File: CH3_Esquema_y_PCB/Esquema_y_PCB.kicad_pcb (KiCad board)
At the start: 2 copper layers, 143.4 x 83.7 mm, 45 parts, among them Q1 BC547, Q10 BC857, Q2 BC547, Q3 BC547, Q4 BC547, Q5 IRF9Z34N, Q7 BC547, Q9 BC857, U1 TL431LP, U2 LM358

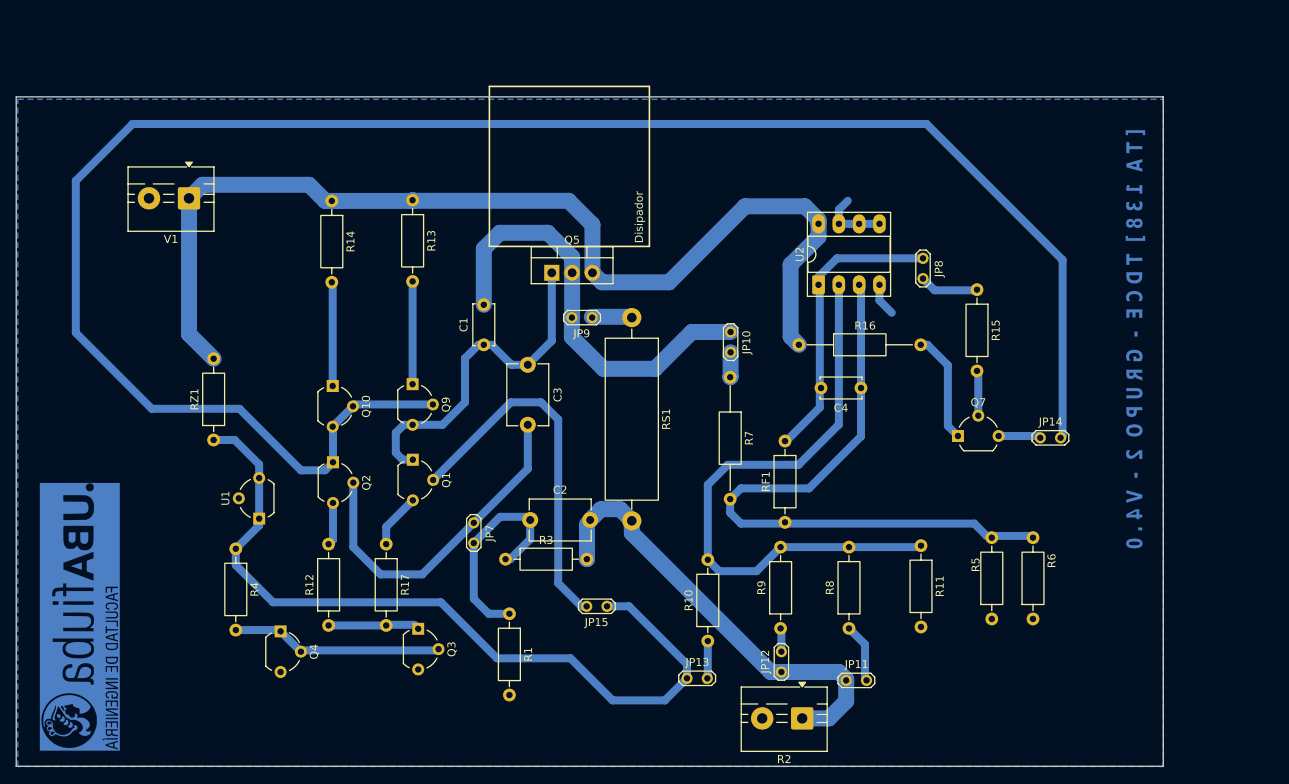
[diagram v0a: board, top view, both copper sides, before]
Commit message: Add files via upload
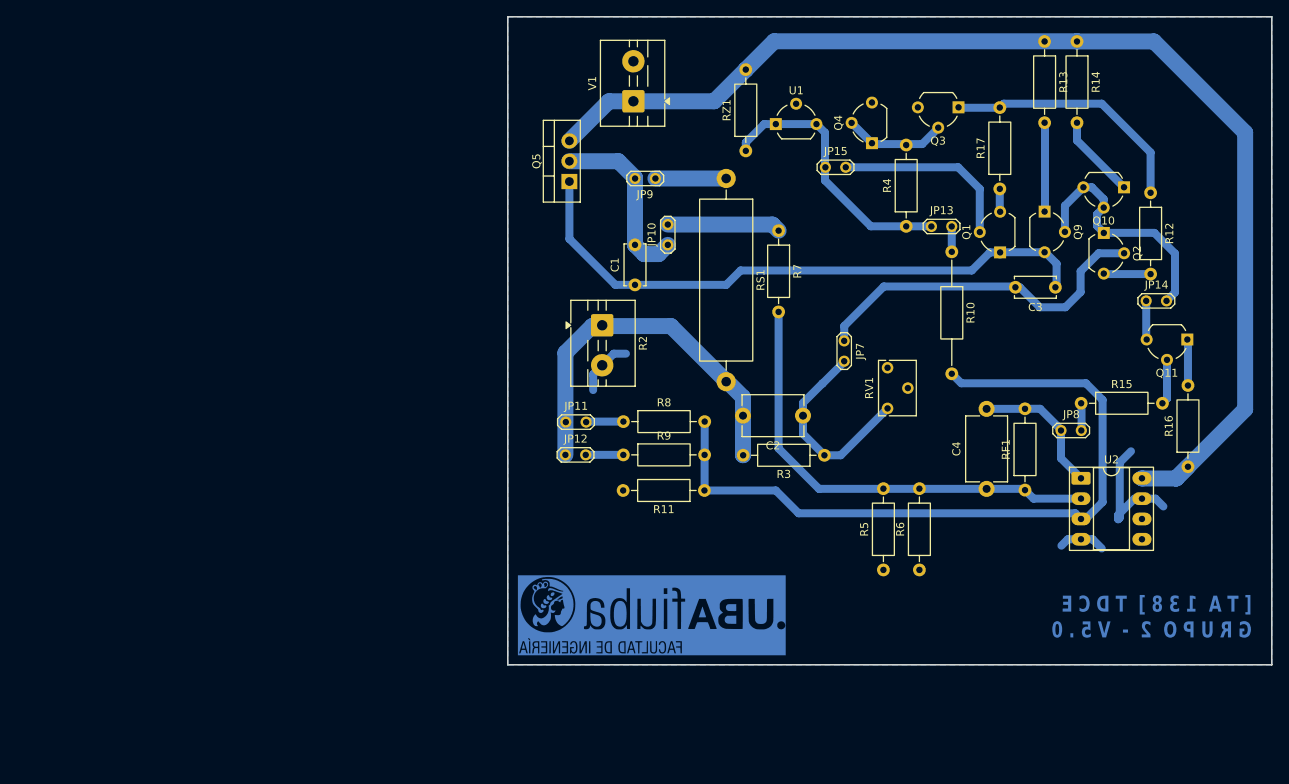
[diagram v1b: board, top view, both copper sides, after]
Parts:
- removed Q7: BC547, Package_TO_SOT_THT:TO-92_Wide
- removed R1: 10k, Resistor_THT:R_Axial_DIN0207_L6.3mm_D2.5mm_P10.16mm_Horizontal
- added Q11: BC557, Package_TO_SOT_THT:TO-92_Wide, F.Cu at (214.9, 90.3)
- added RV1: R_Potentiometer, Potentiometer_THT:Potentiometer_Bourns_3266W_Vertical, F.Cu at (177.5, 93.9)
- C3: footprint Capacitor_THT:C_Disc_D7.5mm_W5.0mm_P7.50mm -> Capacitor_THT:C_Disc_D5.0mm_W2.5mm_P5.00mm
- C4: footprint Capacitor_THT:C_Disc_D5.0mm_W2.5mm_P5.00mm -> Capacitor_THT:C_Disc_D8.0mm_W5.0mm_P10.00mm
- Q10, Q9: value BC857 -> BC557
- R10: footprint Resistor_THT:R_Axial_DIN0207_L6.3mm_D2.5mm_P10.16mm_Horizontal -> Resistor_THT:R_Axial_DIN0207_L6.3mm_D2.5mm_P15.24mm_Horizontal
- R16, R7: footprint Resistor_THT:R_Axial_DIN0207_L6.3mm_D2.5mm_P15.24mm_Horizontal -> Resistor_THT:R_Axial_DIN0207_L6.3mm_D2.5mm_P10.16mm_Horizontal
- moved R12 116.1 mm to (210.3, 72.0), turned to -90 degrees
- moved Q10 102.0 mm to (207.0, 71.3), turned to 180 degrees
- moved Q2 100.5 mm to (204.5, 77.0)
- moved Q4 95.9 mm to (175.5, 65.8), turned to 90 degrees
- moved R14 95.3 mm to (201.2, 53.1)
- moved Q3 93.9 mm to (186.3, 61.3), turned to 180 degrees
- moved R4 93.0 mm to (179.8, 76.2), turned to 90 degrees
- moved R17 88.6 mm to (191.5, 71.5), turned to 90 degrees
- moved Q9 81.9 mm to (197.1, 74.3)
- moved R13 81.5 mm to (197.1, 53.1)
- moved U1 81.3 mm to (163.5, 63.4), turned to 0 degrees
- moved Q1 77.8 mm to (191.5, 79.5), turned to 90 degrees
- moved RZ1 75.7 mm to (159.8, 66.8)
- moved G*** 71.5 mm to (148.0, 124.8), turned to 180 degrees
- moved C3 66.7 mm to (198.4, 83.8), turned to 180 degrees
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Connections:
- C4 pad 1: Net-(U2A-+) -> Net-(U2A--)
- R10 pad 2: Net-(U2A--) -> Net-(U2A-+)
- R11 pad 1: Net-(U2A--) -> Net-(U2A-+)
- R5 pad 2: Net-(U2A-+) -> Net-(U2A--)
- R6 pad 2: Net-(U2A-+) -> Net-(U2A--)
- R7 pad 2: Net-(U2A-+) -> Net-(U2A--)
- R8 pad 2: Net-(U2A--) -> Net-(U2A-+)
- R9 pad 2: Net-(U2A--) -> Net-(U2A-+)
- RF1 pad 1: Net-(U2A-+) -> Net-(U2A--)
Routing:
- net /VB: track 232.5 -> 30.9 mm
- net /in: track 100.0 -> 34.0 mm
- net Net-(Q1-C): track 43.1 -> 76.0 mm
- net /drain: track 53.6 -> 22.5 mm
- net Net-(JP15-B): track 45.8 -> 23.2 mm
- net Net-(Q3-C): track 11.4 -> 32.0 mm
- net Net-(JP8-A): track 36.5 -> 17.5 mm
- net Net-(U2A--): track 74.9 -> 57.5 mm
- net GND: track 12.6 -> 29.6 mm
- net VCC: track 131.5 -> 147.5 mm
- net Net-(U2A-+): track 79.5 -> 93.7 mm
- net Net-(Q3-B): track 26.5 -> 12.7 mm
- net Net-(JP10-B): track 3.13 -> 14.2 mm
- net /out: track 56.9 -> 47.3 mm
- net Net-(Q11-E): track 13.8 -> 5.77 mm
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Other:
- board size 143.4 x 83.7 mm -> 95.5 x 81 mm
- board text added: "[ T A 1 3 8 ] T D C E G R U P O 2 - V 5 . 0"
- board text removed: "[ T A 1 3 8 ] T D C E - G R U P O 2 - V 4 . 0"

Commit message: Add files via upload
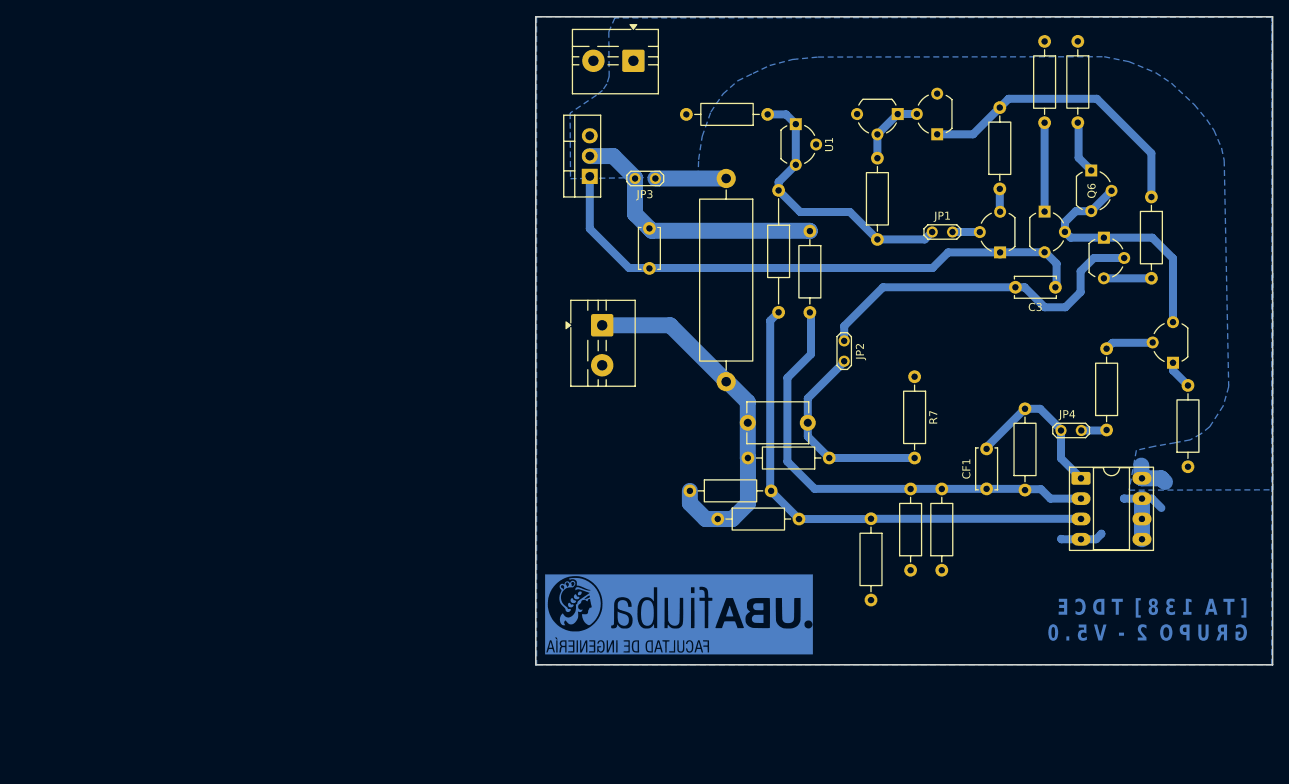
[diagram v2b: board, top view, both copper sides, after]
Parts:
- removed JP10, JP11, JP12, JP13, JP14: Jumper_2_Bridged, TestPoint:TestPoint_2Pads_Pitch2.54mm_Drill0.8mm
- removed RV1: R_Potentiometer, Potentiometer_THT:Potentiometer_Bourns_3266W_Vertical
- added R7: 5k1, Resistor_THT:R_Axial_DIN0207_L6.3mm_D2.5mm_P10.16mm_Horizontal, F.Cu at (180.8, 95.0)
- C2: value 820p -> 1.2n
- CF1: renamed from C4; footprint Capacitor_THT:C_Disc_D8.0mm_W5.0mm_P10.00mm -> Capacitor_THT:C_Disc_D5.0mm_W2.5mm_P5.00mm
- R1: renamed from R17; value 2k2 -> 1k
- R2: renamed from R12; value 2k2 -> 1k
- R6: renamed from R3; value 10k -> 5k1
- moved R13 23.0 mm to (163.8, 71.7)
- moved R14 21.1 mm to (175.4, 112.7), turned to -90 degrees
- moved R11 17.0 mm to (156.2, 112.8)
- moved JP1 15.6 mm to (183.1, 76.9)
- moved R12 9.46 mm to (152.8, 109.3)
- moved RZ1 5.31 mm to (162.5, 62.2), turned to 180 degrees
- moved V1 5.06 mm to (145.7, 55.5), turned to 180 degrees
- moved Q4 4.86 mm to (178.7, 62.2), turned to 180 degrees
- moved R15 4.61 mm to (204.8, 101.7), turned to 90 degrees
- moved Q6 4.61 mm to (202.9, 69.2), turned to -90 degrees
- moved Q3 4.30 mm to (183.7, 64.7), turned to 90 degrees
- moved R3 3.96 mm to (176.2, 77.8)
- moved R10 3.91 mm to (167.8, 76.8)
- moved Q7 3.42 mm to (213.2, 93.2), turned to 90 degrees
- moved G*** 3.40 mm to (151.4, 124.7)
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- renumbered JP15 to JP1, JP7 to JP2, JP9 to JP3, JP8 to JP4, Q5 to MOS1, Q9 to Q5, Q10 to Q6, Q11 to Q7, R7 to R10, R8 to R11, R9 to R12, R10 to R13, R11 to R14, R4 to R3, R13 to R4, R14 to R5, R5 to R8, R6 to R9, R2 to RL1
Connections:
- Q7 pad 3: Net-(JP14-A) -> /VB
- R10 pad 1: Net-(JP10-B) -> /drain
- R11 pad 1: Net-(JP11-B) -> /out
- R12 pad 1: Net-(JP12-B) -> /out
- R13 pad 1: Net-(JP13-B) -> /in
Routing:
- net VCC: track 147.5 -> 4.69 mm
- net Net-(U2A-+): track 93.7 -> 63.5 mm
- net Net-(JP1-B): track 23.2 -> 3.41 mm
- net Net-(JP10-B): track 14.2 -> 0.00 mm
- net GND: track 29.6 -> 15.7 mm
- net /drain: track 22.5 -> 34.0 mm
- net Net-(Q3-C): track 32.0 -> 36.9 mm
- net Net-(JP14-A): track 4.85 -> 0.00 mm
- net Net-(JP12-B): track 4.71 -> 0.00 mm
- net Net-(JP11-B): track 4.68 -> 0.00 mm
- net Net-(MOS1-G): track 76.0 -> 71.6 mm
- net Net-(Q6-E): track 10.5 -> 6.71 mm
- net Net-(Q3-B): track 12.7 -> 8.96 mm
- net Net-(JP13-B): track 3.17 -> 0.00 mm
- net Net-(JP4-A): track 17.5 -> 19.7 mm
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- added copper zone on B.Cu, net VCC
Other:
- board size 95.5 x 81 mm -> 92.1 x 81 mm
